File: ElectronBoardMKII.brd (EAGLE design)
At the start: 84 x 200 mm, 59 parts, among them IC1 7805TV, K1 AQYAQY27, Q1 BSS170, Q2 BSS170, U1 LM386N

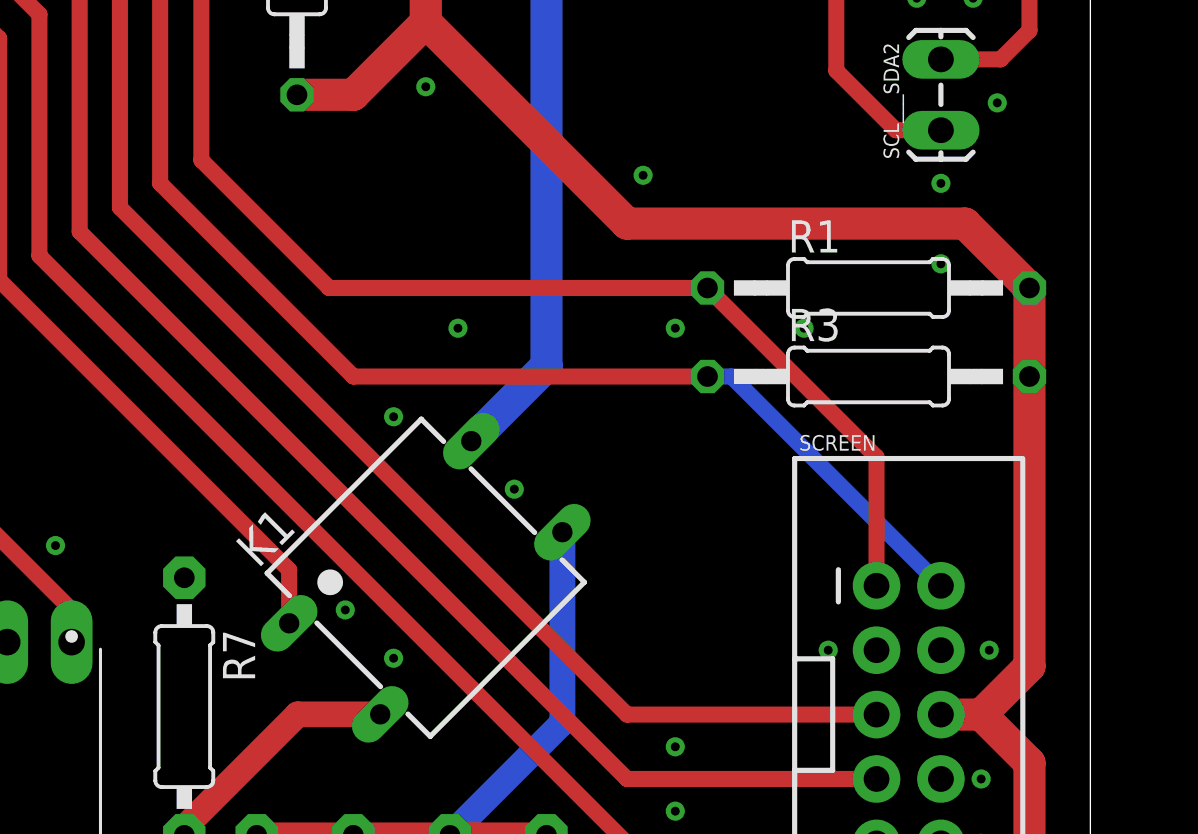
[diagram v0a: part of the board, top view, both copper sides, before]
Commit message: Update
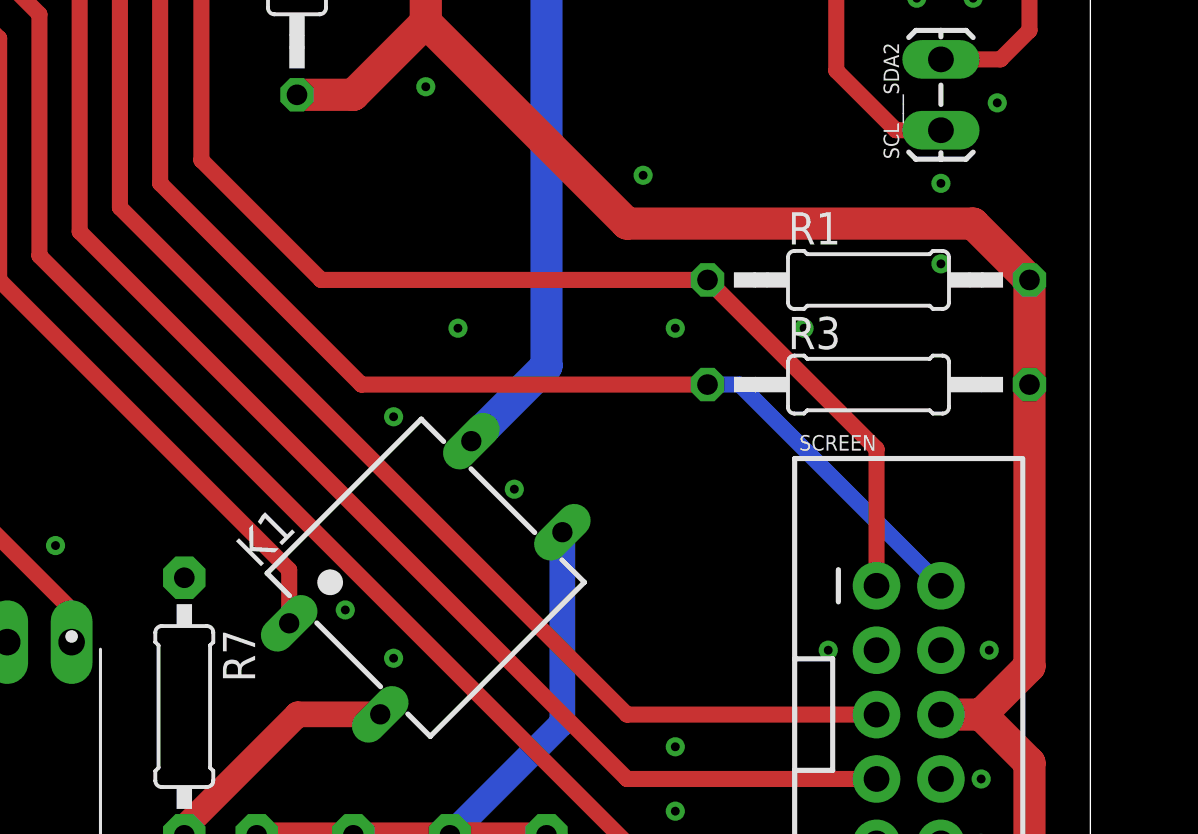
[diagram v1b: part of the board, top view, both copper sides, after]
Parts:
- moved R1 0.32 mm to (75.2, 70.2)
- moved R3 0.32 mm to (75.2, 66.0)
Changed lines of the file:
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@@
 <attribute name="VALUE" x="3.1115" y="93.218" size="0.6096" layer="27" font="vector" ratio="20" rot="R270"/>
 </element>
-<element name="R1" library="resistor" library_urn="urn:adsk.eagle:library:348" package="0207/12" package3d_urn="urn:adsk.eagle:package:23489/1" value="4.7k" x="75.2475" y="69.85">
-<attribute name="NAME" x="72.0725" y="71.247" size="1.27" layer="25" ratio="10"/>
-<attribute name="VALUE" x="72.9615" y="69.1642" size="1.27" layer="27" ratio="10"/>
-</element>
-<element name="R3" library="resistor" library_urn="urn:adsk.eagle:library:348" package="0207/12" package3d_urn="urn:adsk.eagle:package:23489/1" value="4.7k" x="75.2475" y="66.3575">
-<attribute name="NAME" x="72.0725" y="67.7545" size="1.27" layer="25" ratio="10"/>
-<attribute name="VALUE" x="72.9615" y="65.6717" size="1.27" layer="27" ratio="10"/>
+<element name="R1" library="resistor" library_urn="urn:adsk.eagle:library:348" package="0207/12" package3d_urn="urn:adsk.eagle:package:23489/1" value="4.7k" x="75.2475" y="70.1675">
+<attribute name="NAME" x="72.0725" y="71.5645" size="1.27" layer="25" ratio="10"/>
+<attribute name="VALUE" x="72.9615" y="69.4817" size="1.27" layer="27" ratio="10"/>
+</element>
+<element name="R3" library="resistor" library_urn="urn:adsk.eagle:library:348" package="0207/12" package3d_urn="urn:adsk.eagle:package:23489/1" value="4.7k" x="75.2475" y="66.04">
+<attribute name="NAME" x="72.0725" y="67.437" size="1.27" layer="25" ratio="10"/>
+<attribute name="VALUE" x="72.9615" y="65.3542" size="1.27" layer="27" ratio="10"/>
 </element>
 <element name="R16" library="resistor" library_urn="urn:adsk.eagle:library:348" package="0207/12" package3d_urn="urn:adsk.eagle:package:23489/1" value="47k" x="36.195" y="71.12" rot="R90">
@@
 <contactref element="SCREEN" pad="2"/>
 <contactref element="R3" pad="1"/>
-<wire x1="68.8975" y1="66.3575" x2="69.85" y2="66.3575" width="0.635" layer="16"/>
-<wire x1="69.85" y1="66.3575" x2="78.105" y2="58.1025" width="0.635" layer="16"/>
+<wire x1="68.8975" y1="66.04" x2="70.1675" y2="66.04" width="0.635" layer="16"/>
+<wire x1="70.1675" y1="66.04" x2="78.105" y2="58.1025" width="0.635" layer="16"/>
 <wire x1="39.37" y1="91.44" x2="47.3075" y2="83.5025" width="0.635" layer="1"/>
 <wire x1="47.3075" y1="83.5025" x2="47.3075" y2="73.9775" width="0.635" layer="1"/>
-<wire x1="47.3075" y1="73.9775" x2="54.9275" y2="66.3575" width="0.635" layer="1"/>
-<wire x1="54.9275" y1="66.3575" x2="68.8975" y2="66.3575" width="0.635" layer="1"/>
+<wire x1="47.3075" y1="73.9775" x2="55.245" y2="66.04" width="0.635" layer="1"/>
+<wire x1="55.245" y1="66.04" x2="68.8975" y2="66.04" width="0.635" layer="1"/>
 <contactref element="J4" pad="5"/>
 <wire x1="37.2745" y1="91.44" x2="39.37" y2="91.44" width="0.635" layer="1"/>
@@
 <contactref element="SCREEN" pad="1"/>
 <contactref element="R1" pad="1"/>
-<wire x1="75.565" y1="58.1025" x2="75.565" y2="63.1825" width="0.635" layer="1"/>
-<wire x1="75.565" y1="63.1825" x2="68.8975" y2="69.85" width="0.635" layer="1"/>
-<wire x1="68.8975" y1="69.85" x2="53.975" y2="69.85" width="0.635" layer="1"/>
+<wire x1="75.565" y1="58.1025" x2="75.565" y2="63.5" width="0.635" layer="1"/>
+<wire x1="75.565" y1="63.5" x2="68.8975" y2="70.1675" width="0.635" layer="1"/>
+<wire x1="68.8975" y1="70.1675" x2="53.6575" y2="70.1675" width="0.635" layer="1"/>
 <wire x1="39.37" y1="93.98" x2="48.9331" y2="84.4169" width="0.635" layer="1"/>
-<wire x1="53.975" y1="69.85" x2="48.9331" y2="74.8919" width="0.635" layer="1"/>
+<wire x1="53.6575" y1="70.1675" x2="48.9331" y2="74.8919" width="0.635" layer="1"/>
 <wire x1="48.9331" y1="74.8919" x2="48.9331" y2="84.4169" width="0.635" layer="1"/>
 <contactref element="J4" pad="4"/>
@@
 <wire x1="78.105" y1="53.0225" x2="79.6925" y2="53.0225" width="1.27" layer="1"/>
 <wire x1="79.6925" y1="53.0225" x2="81.5975" y2="54.9275" width="1.27" layer="1"/>
-<wire x1="81.5975" y1="54.9275" x2="81.5975" y2="66.3575" width="1.27" layer="1"/>
-<wire x1="81.5975" y1="66.3575" x2="81.5975" y2="69.85" width="1.27" layer="1"/>
+<wire x1="81.5975" y1="54.9275" x2="81.5975" y2="66.04" width="1.27" layer="1"/>
+<wire x1="81.5975" y1="66.04" x2="81.5975" y2="70.1675" width="1.27" layer="1"/>
 <wire x1="52.705" y1="77.47" x2="54.9275" y2="77.47" width="1.27" layer="1"/>
 <wire x1="54.9275" y1="77.47" x2="57.785" y2="80.3275" width="1.27" layer="1"/>
 <wire x1="57.785" y1="80.3275" x2="57.785" y2="81.915" width="1.27" layer="1"/>
 <wire x1="57.785" y1="80.3275" x2="65.7225" y2="72.39" width="1.27" layer="1"/>
-<wire x1="65.7225" y1="72.39" x2="79.0575" y2="72.39" width="1.27" layer="1"/>
-<wire x1="79.0575" y1="72.39" x2="81.5975" y2="69.85" width="1.27" layer="1"/>
+<wire x1="65.7225" y1="72.39" x2="79.375" y2="72.39" width="1.27" layer="1"/>
+<wire x1="79.375" y1="72.39" x2="81.5975" y2="70.1675" width="1.27" layer="1"/>
 <wire x1="81.5975" y1="46.99" x2="81.5975" y2="51.1175" width="1.27" layer="1"/>
 <wire x1="81.5975" y1="51.1175" x2="79.6925" y2="53.0225" width="1.27" layer="1"/>
